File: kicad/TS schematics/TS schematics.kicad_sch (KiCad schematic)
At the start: 13 parts, among them J1 Conn_01x05, J2 TSAL_R, J4 TSMP, K1 DISCHARGE RELAY GIGAVAC PNC11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

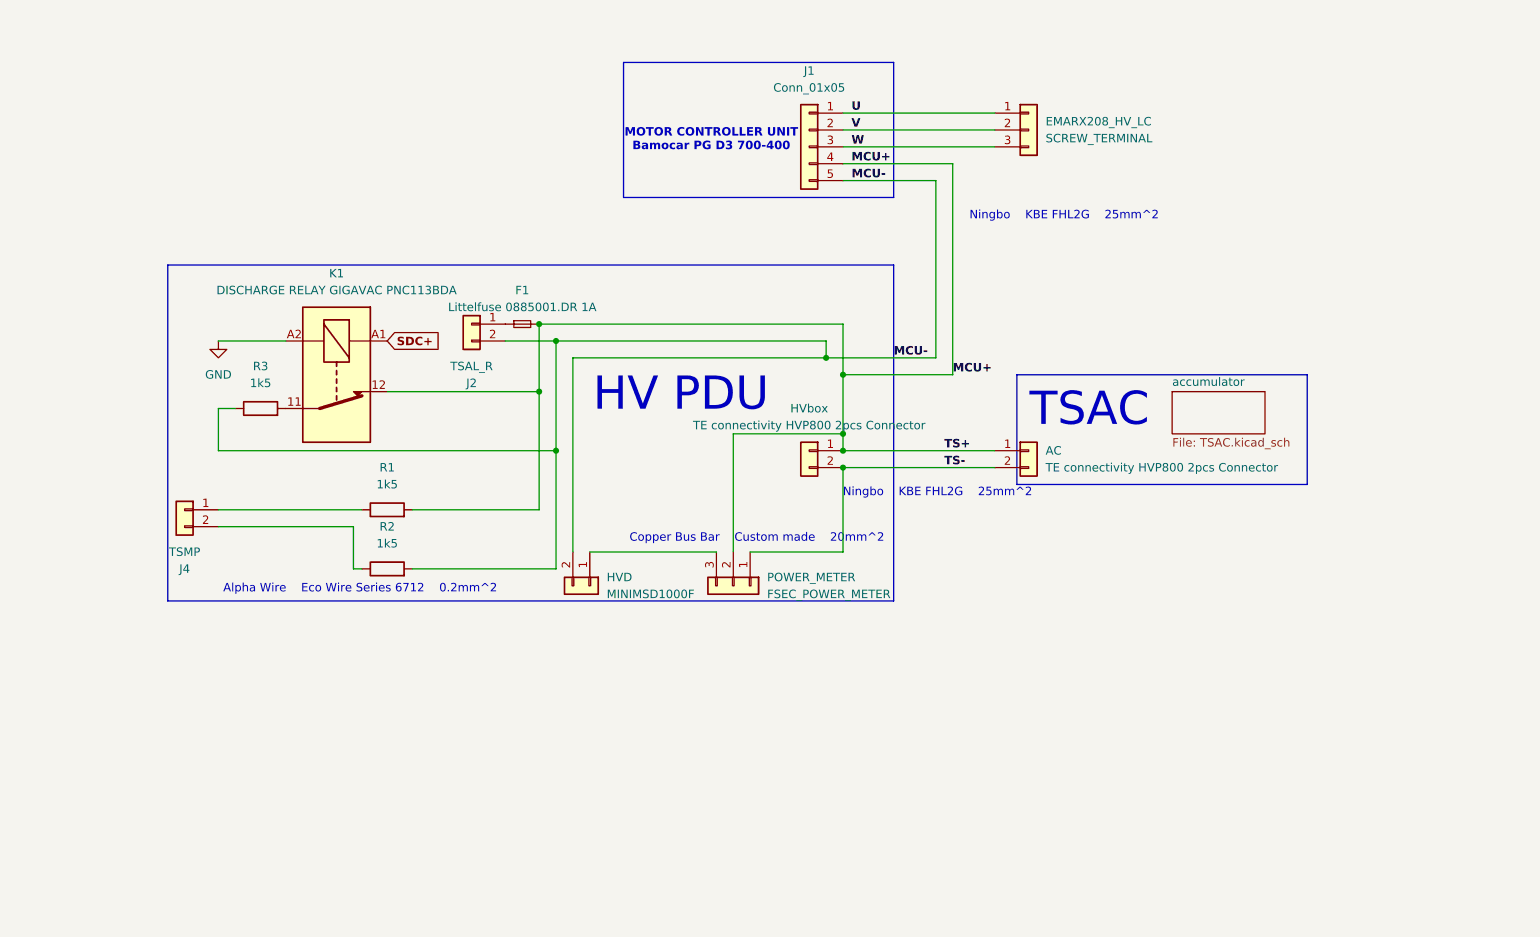
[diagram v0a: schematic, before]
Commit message: new schematics
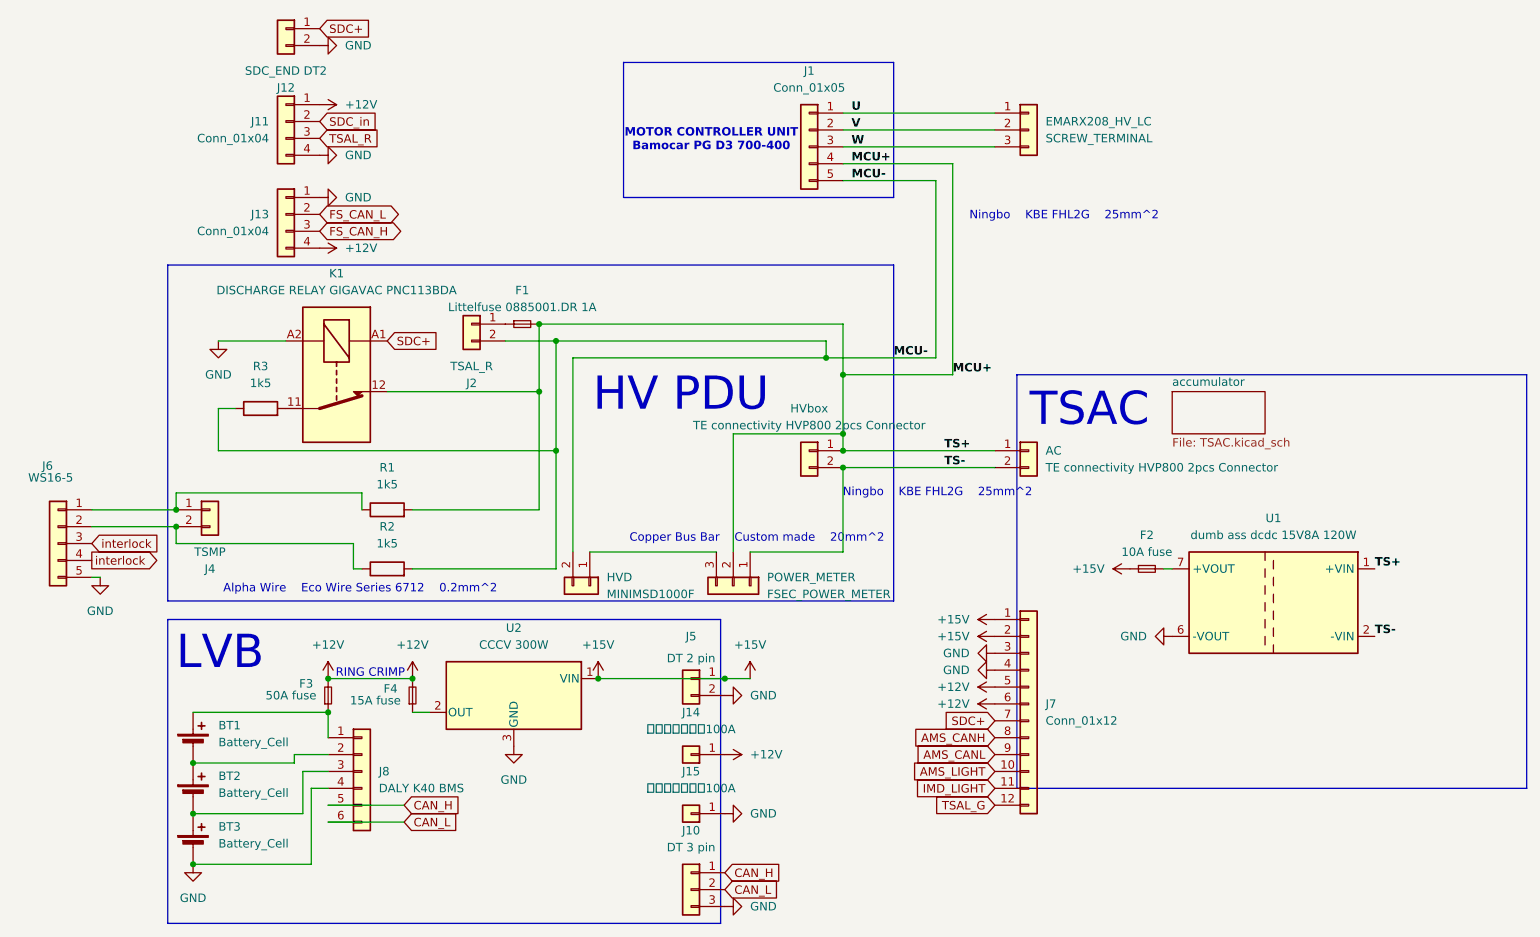
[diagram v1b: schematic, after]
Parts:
- added BT1, BT2, BT3: Battery_Cell, symbol Device:Battery_Cell
- added F2: 10A fuse, symbol Device:Fuse_Small
- added F3: 50A fuse, symbol Device:Fuse_Small
- added F4: 15A fuse, symbol Device:Fuse_Small
- added J10: DT 3 pin, symbol Connector_Generic:Conn_01x03
- added J11, J13: Conn_01x04, symbol Connector_Generic:Conn_01x04
- added J12: SDC_END DT2, symbol Connector_Generic:Conn_01x02
- added J14: 紅色儲能接綫柱100A, symbol Connector_Generic:Conn_01x01
- added J15: 黑色儲能接綫柱100A, symbol Connector_Generic:Conn_01x01
- added J5: DT 2 pin, symbol Connector_Generic:Conn_01x02
- added J6: WS16-5, symbol Connector_Generic:Conn_01x05
- added J7: Conn_01x12, symbol Connector_Generic:Conn_01x12
- added J8: DALY K40 BMS, symbol Connector_Generic:Conn_01x06
- added U1: dumb ass dcdc 15V8A 120W, Converter_DCDC:Converter_DCDC_TRACO_TDN_5-xxxxWISM_SMD, symbol Regulator_Switching:TDN_5-0910WISM
- added U2: CCCV 300W, Package_TO_SOT_THT:TO-220-5_Vertical, symbol Regulator_Switching:LM2575-12BT
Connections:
- net GND: now also BT3.2 (-), J10.3 (Pin_3), J11.4 (Pin_4), J12.2 (Pin_2), J13.1 (Pin_1), J15.1 (Pin_1), J5.2 (Pin_2), J6.5 (Pin_5), J7.3 (Pin_3), J7.4 (Pin_4), J8.4 (Pin_4), U1.6 (-VOUT), U2.3 (GND)
- net MCU+: now also U1.1 (+VIN)
- net SDC+: now also J12.1 (Pin_1), J7.7 (Pin_7)
- net TS-: now also U1.2 (-VIN)
- net at J4.1 (Pin_1), R1.1: now also J6.1 (Pin_1)
- net at J4.2 (Pin_2), R2.1: now also J6.2 (Pin_2)
- new net: BT1.2 (-), BT2.1 (+), J8.2 (Pin_2)
- new net: BT2.2 (-), BT3.1 (+), J8.3 (Pin_3)
- new net: F4.1, U2.2 (OUT)
- new net: F2.2, U1.7 (+VOUT)
- new net: BT1.1 (+), F3.1, J8.1 (Pin_1)
- new net +12V: F3.2, F4.2, J11.1 (Pin_1), J13.4 (Pin_4), J14.1 (Pin_1), J7.5 (Pin_5), J7.6 (Pin_6)
- new net +15V: F2.1, J5.1 (Pin_1), J7.1 (Pin_1), J7.2 (Pin_2), U2.1 (VIN)
- new net AMS_CANH: J7.8 (Pin_8)
- new net AMS_CANL: J7.9 (Pin_9)
- new net AMS_LIGHT: J7.10 (Pin_10)
- new net CAN_H: J10.1 (Pin_1), J8.5 (Pin_5)
- new net CAN_L: J10.2 (Pin_2), J8.6 (Pin_6)
- new net FS_CAN_H: J13.3 (Pin_3)
- new net FS_CAN_L: J13.2 (Pin_2)
- new net IMD_LIGHT: J7.11 (Pin_11)
- new net SDC_in: J11.2 (Pin_2)
- new net TSAL_G: J7.12 (Pin_12)
- new net TSAL_R: J11.3 (Pin_3)
- new net interlock: J6.3 (Pin_3), J6.4 (Pin_4)
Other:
- note added: "LVB"
- note added: "RING CRIMP"
